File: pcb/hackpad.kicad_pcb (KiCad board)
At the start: 2 copper layers, 41 x 62.5 mm, 7 parts, among them SW1 SW_Push, SW2 SW_Push, SW3 SW_Push, SW4 SW_Push, U1 XIAO-RP2040-DIP

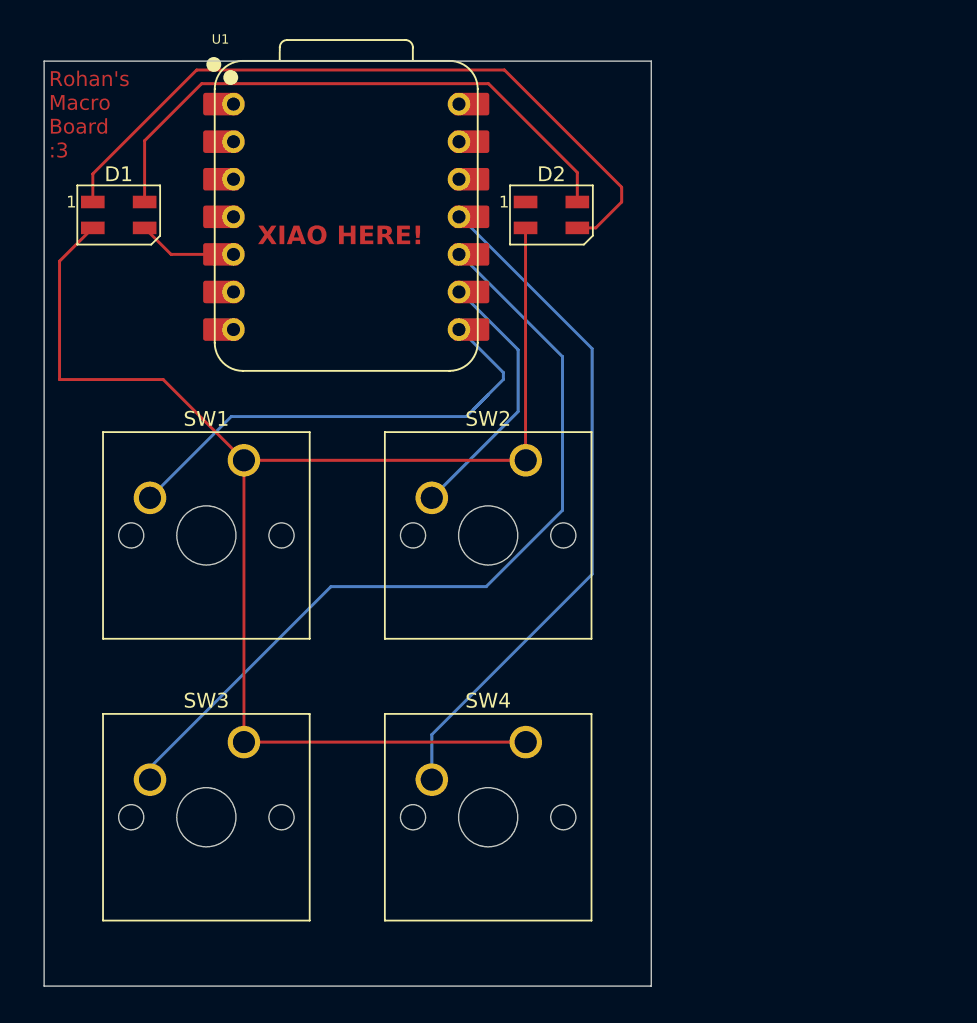
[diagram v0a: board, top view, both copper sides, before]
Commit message: Made the thing actually unique and cool and stuff
yay!
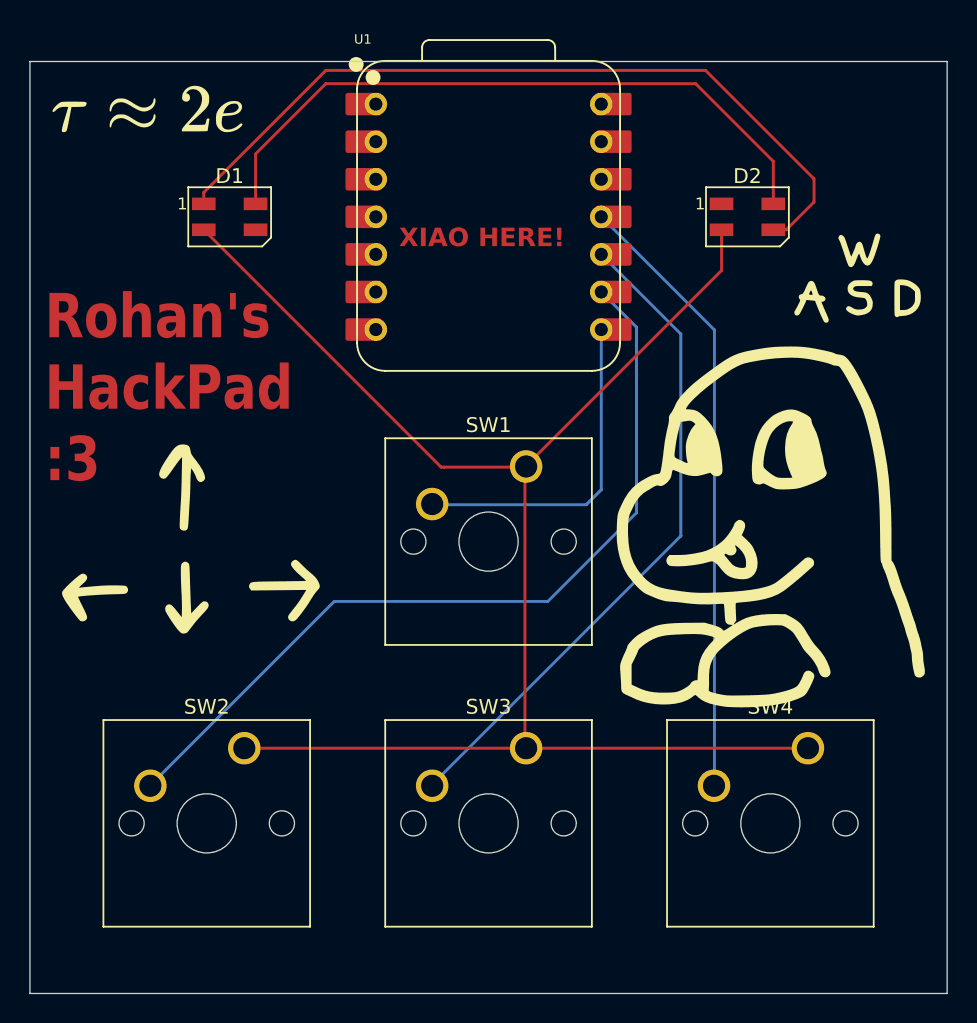
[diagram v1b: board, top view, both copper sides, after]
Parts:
- added G***: LOGO, LOGO, F.Cu at (206.0, 92.0)
- added G***: LOGO, LOGO, F.Cu at (158.0, 81.0)
- added G***: LOGO, LOGO, F.Cu at (200.0, 109.0)
- added G***: LOGO, LOGO, F.Cu at (161.0, 110.0)
- moved SW2 27.2 mm to (164.5, 123.9)
- moved SW1 19.1 mm to (183.5, 104.9)
- moved SW4 19.1 mm to (202.6, 123.9)
- moved SW3 19.1 mm to (183.5, 123.9)
- moved D2 13.3 mm to (198.5, 88.0)
- moved U1 9.62 mm to (181.0, 88.0)
- moved D1 7.50 mm to (163.5, 88.0)
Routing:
- net Net-(U1-GPIO2/SCK): track 18.0 -> 56.4 mm
- net Net-(U1-GPIO4/MISO): track 56.1 -> 45.1 mm
- net Net-(U1-GPIO1/RX): track 33.2 -> 22.8 mm
- net GND: track 98.8 -> 107.0 mm
- net Net-(D1-DIN): track 6.85 -> 0.00 mm
- net +5V: track 39.5 -> 45.4 mm
- net Net-(D1-DOUT): track 48.6 -> 53.6 mm
- net Net-(U1-GPIO3/MOSI): track 46.2 -> 41.6 mm
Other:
- board size 41 x 62.5 mm -> 62 x 63 mm
- board text added: "Rohan's HackPad :3"
- board text removed: "Rohan's Macro Board :3"
